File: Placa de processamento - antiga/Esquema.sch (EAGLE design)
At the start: 12 parts

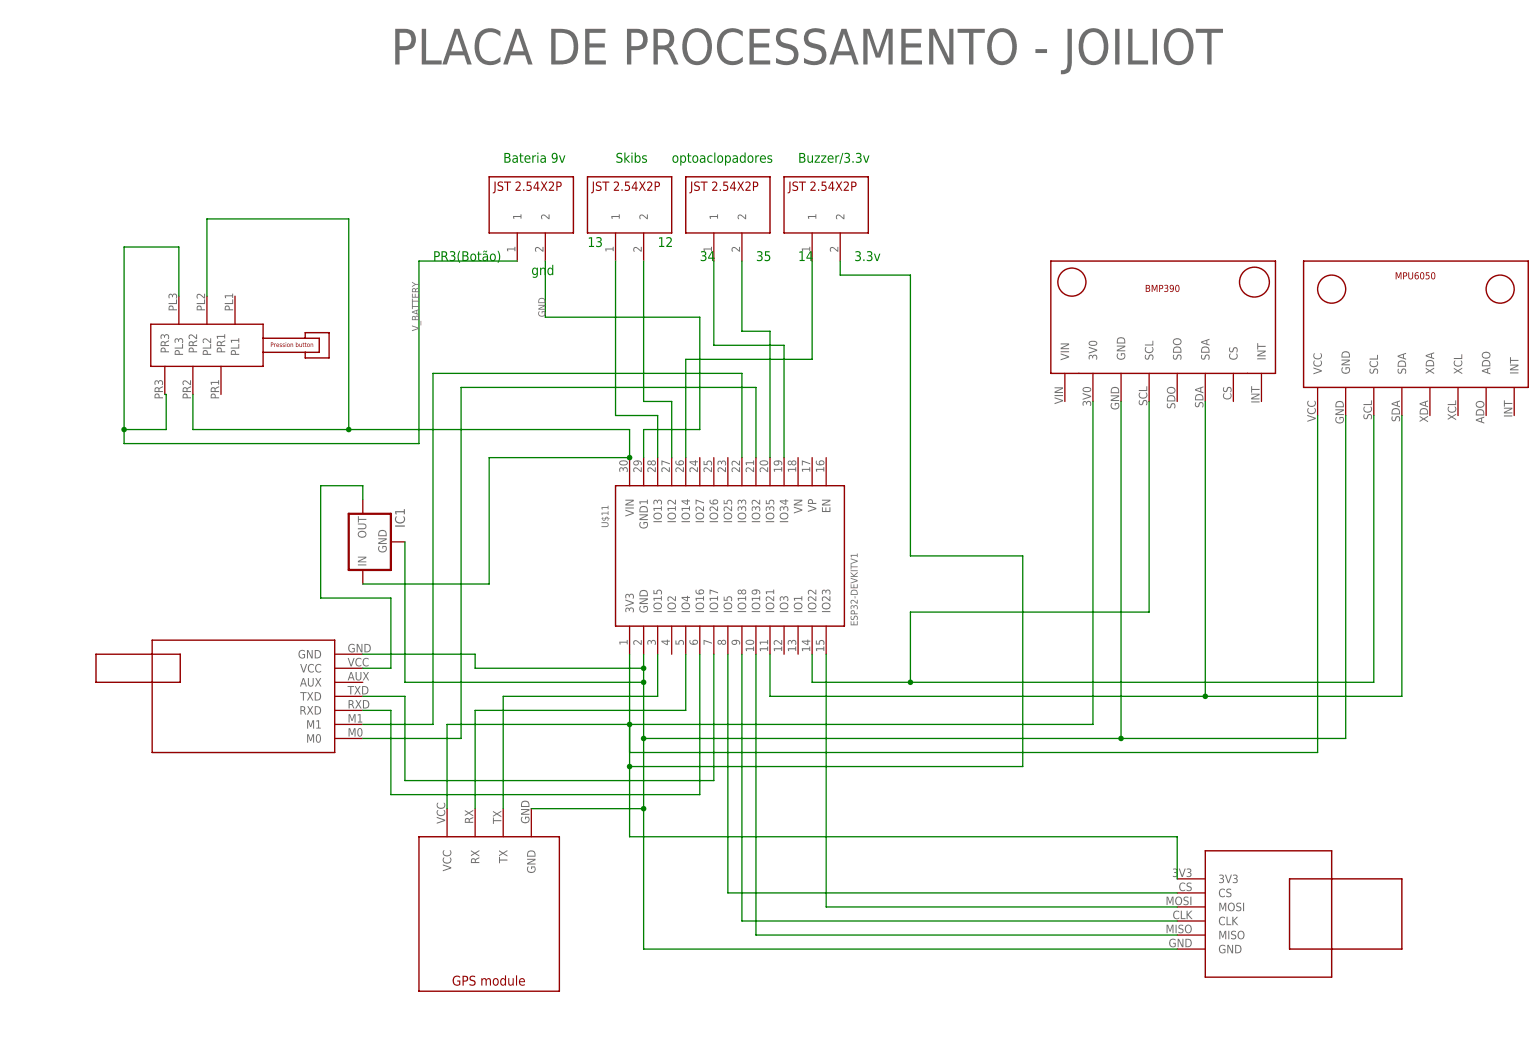
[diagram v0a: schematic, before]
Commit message: Roteamento da placa
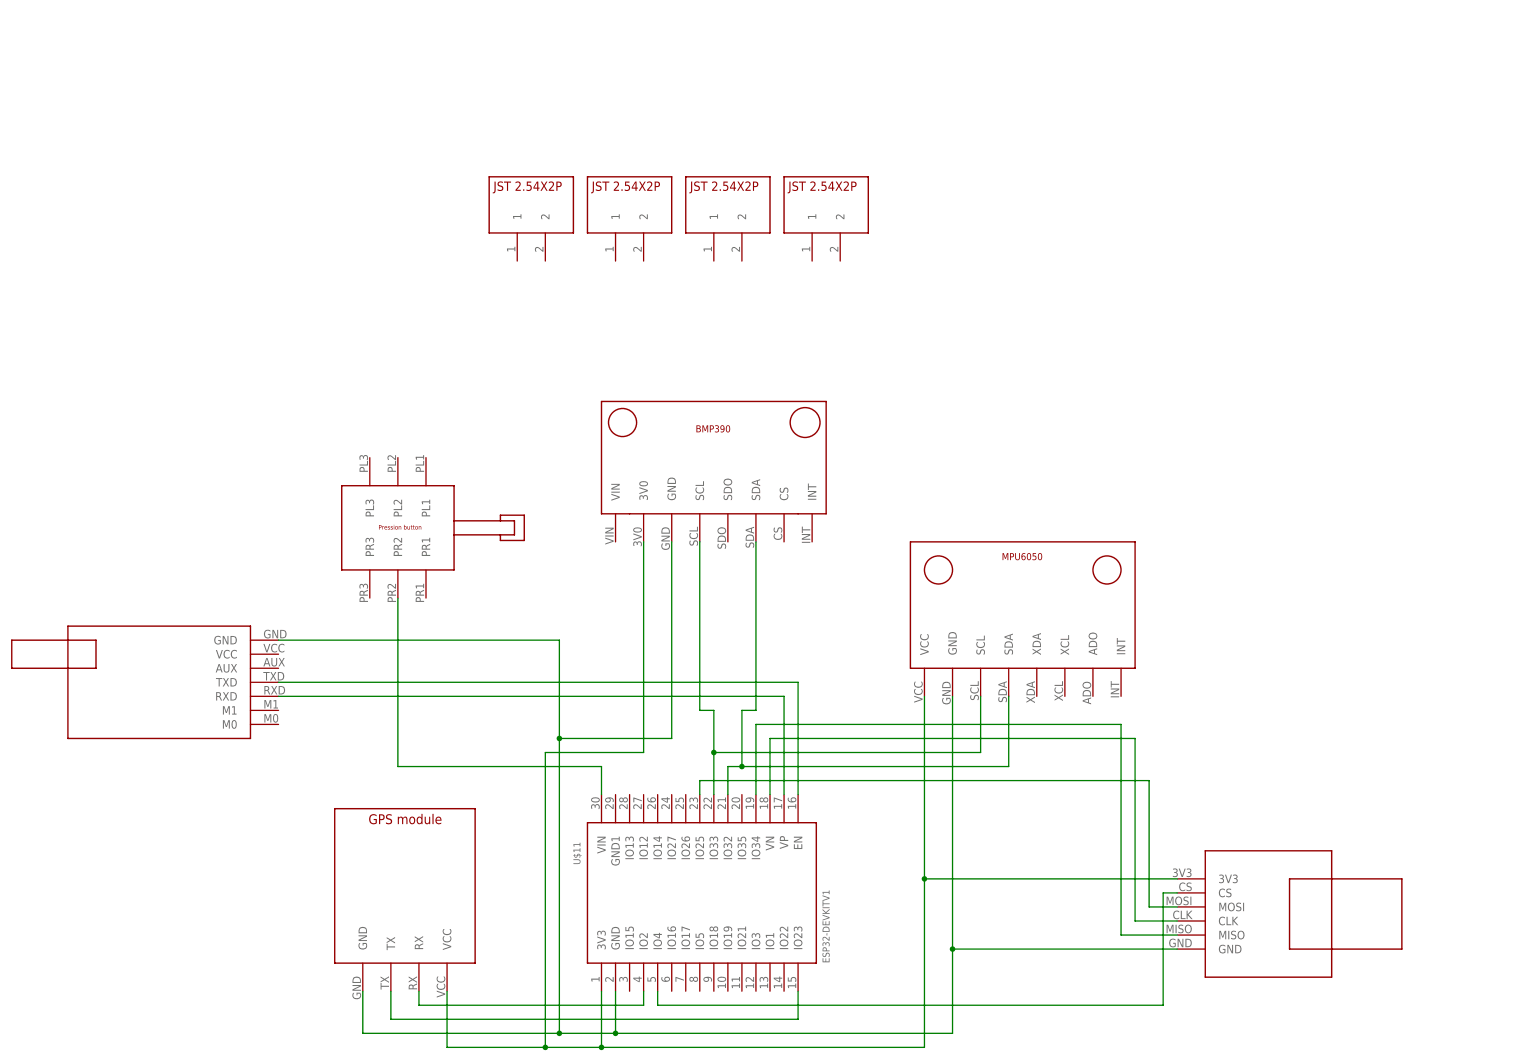
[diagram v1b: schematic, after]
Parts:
- removed IC1: (no value), v-reg:78LXX
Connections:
- removed net GND: U$11.GND1, U$7.2
- removed net N$12: IC1.OUT, U$2.VCC
- removed net N$15: U$11.IO18, U$8.CLK
- removed net N$16: U$11.IO19, U$8.MISO
- removed net N$19: U$11.IO13, U$6.1
- removed net N$20: U$11.IO12, U$6.2
- removed net N$21: U$11.IO14, U$4.1
- removed net N$22: U$11.IO34, U$5.1
- removed net N$23: U$11.IO35, U$5.2
- removed net V_BATTERY: U$10.PL3, U$10.PR3, U$7.1
- net N$1: now also U$11.IO32; no longer U$11.IO21
- net N$10: now also U$11.IO34, U$8.MISO; no longer U$11.IO33, U$2.M1
- net N$11: now also U$10.PR2, U$11.VIN; no longer U$11.IO32, U$2.M0
- net N$13: now also U$11.VP, U$2.RXD; no longer U$11.IO5, U$8.CS
- net N$14: now also U$11.EN, U$2.TXD; no longer U$11.IO23, U$8.MOSI
- net N$2: now also U$11.IO33; no longer U$11.IO22
- net N$3: no longer U$4.2
- net N$4: no longer IC1.GND
- net N$5: now also U$11.IO23, U$3.TX; no longer U$11.IO4, U$3.RX
- net N$6: now also U$11.IO2, U$3.RX; no longer U$11.IO15, U$3.TX
- net N$7: now also U$11.IO4, U$8.CS; no longer IC1.IN, U$10.PL2, U$10.PR2, U$11.VIN
- net N$8: now also U$11.IO25, U$8.MOSI; no longer U$11.IO17, U$2.TXD
- net N$9: now also U$11.VN, U$8.CLK; no longer U$11.IO16, U$2.RXD
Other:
- note removed: "12"
- note removed: "13"
- note removed: "14"
- note removed: "3.3v"
- note removed: "34"
- note removed: "35"
- note removed: "Bateria 9v"
- note removed: "Buzzer/3.3v"
- note removed: "PLACA DE PROCESSAMENTO - JOILIOT"
- note removed: "PR3(Botão)"
- note removed: "Skibs"
- note removed: "gnd"
- note removed: "optoaclopadores"
- moved on the sheet: U$11
